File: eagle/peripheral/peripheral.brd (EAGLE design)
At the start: 160 x 100 mm, 0 parts

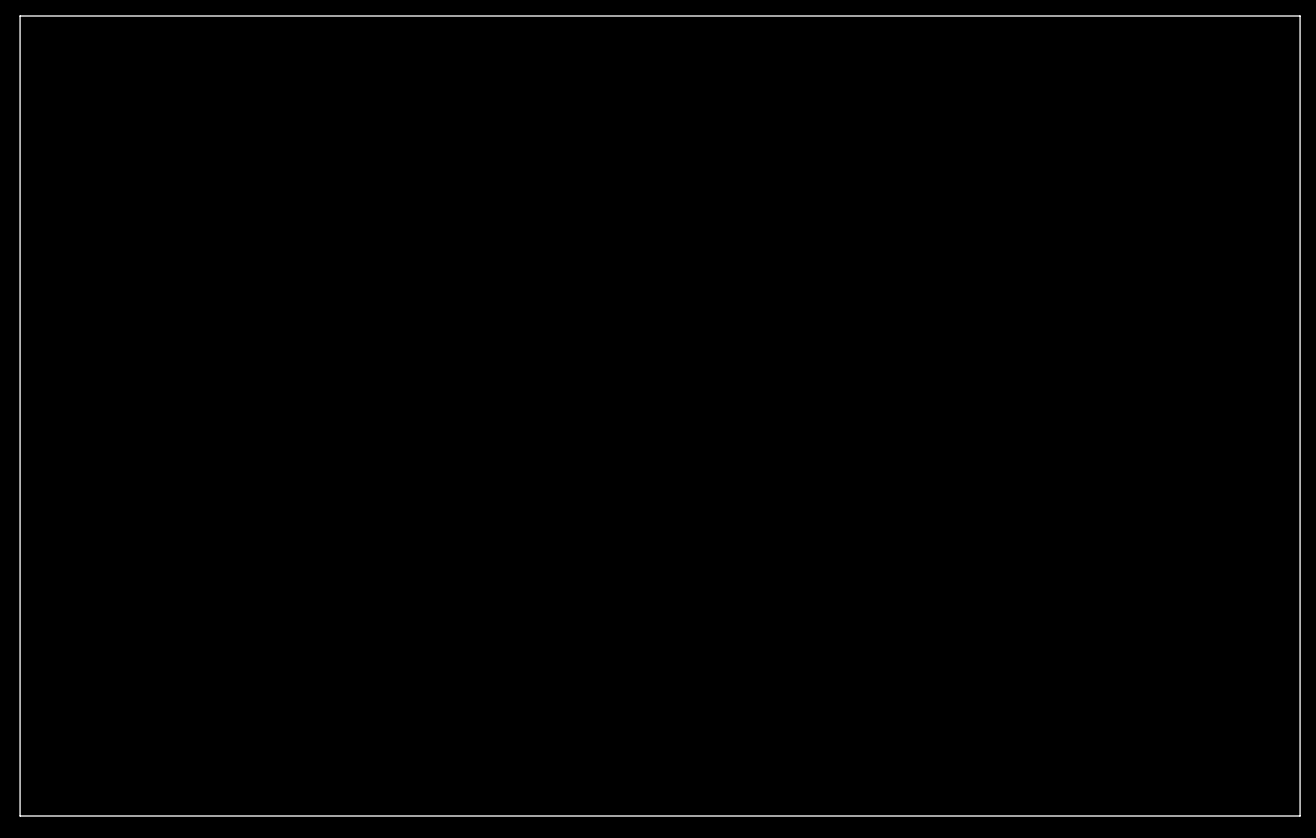
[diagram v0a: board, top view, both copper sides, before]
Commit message: Completed peripheral design layout.
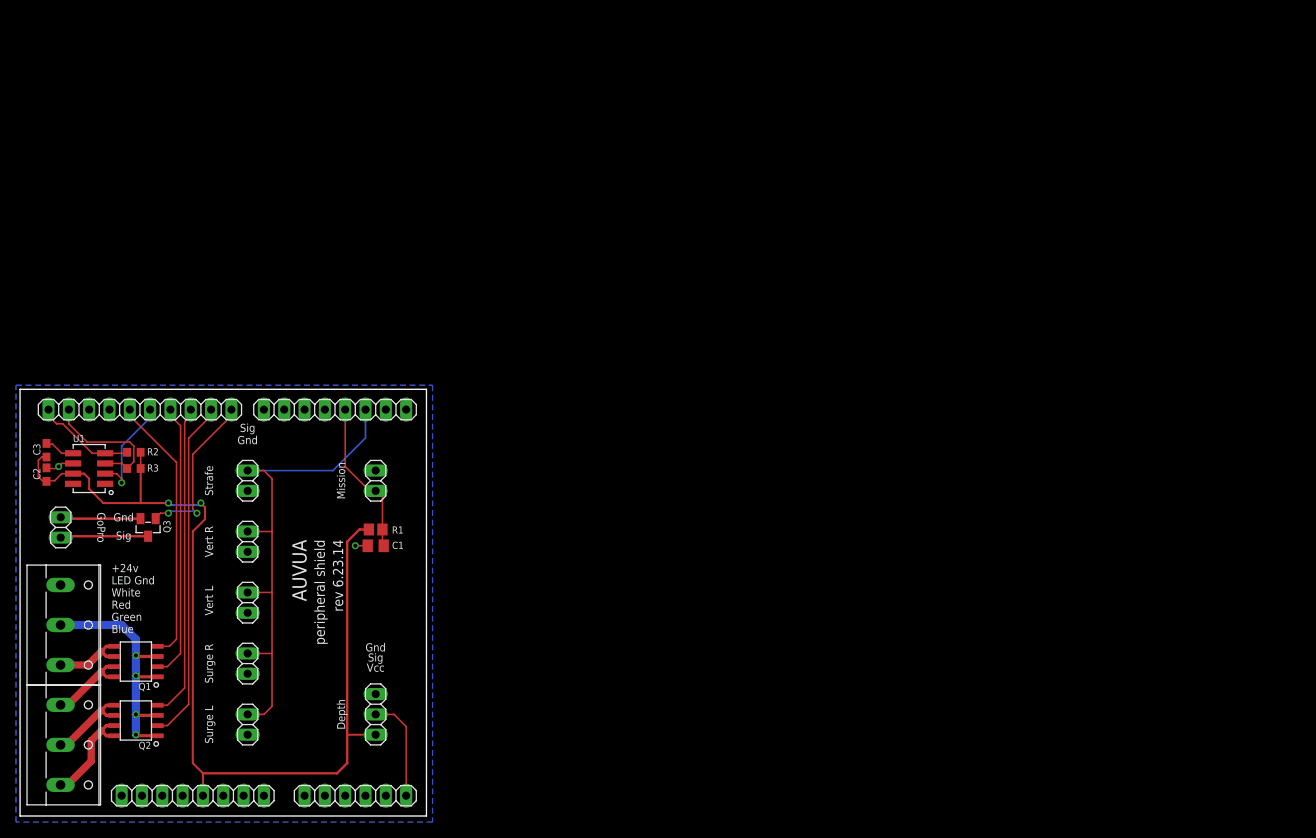
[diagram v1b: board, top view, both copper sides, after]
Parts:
- added C1: 10u, resistor:C0805K
- added C2: 220n, resistor:C0603
- added C3: 100n, resistor:C0603
- added JP1: (no value), pinhead:1X10
- added JP10, JP11, JP5, JP6, JP7, JP8, JP9: (no value), pinhead:1X02
- added JP12: (no value), pinhead:1X03
- added JP2, JP3: (no value), pinhead:1X08
- added JP4: (no value), pinhead:1X06
- added Q1, Q2: DMN4031SSD, peripheral:SO-8
- added Q3: BSS123, peripheral:SOT-23
- added R1: 100k, resistor:R0805
- added R2, R3: 4.7k, resistor:R0603
- added U1: CHIPCAP2, peripheral:CHIPCAP2
- added X1, X2: (no value), con-wago-500:W237-103
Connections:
- new net +24V: X1.1
- new net 0/RX1: JP2.8
- new net 1/TX1: JP2.7
- new net 10: JP1.8, Q2.4
- new net 11: JP1.7, Q1.2
- new net 12: JP1.6, U1.2
- new net 13: JP1.5, Q1.4
- new net 2: JP10.1, JP2.6, JP6.1, JP7.1, JP8.1, JP9.1
- new net 3: C1.1, JP2.5, JP5.1, R1.1
- new net 3.3V: JP3.4
- new net 4: JP2.4
- new net 5: JP2.3
- new net 5V: C2.1, C3.1, JP12.1, JP3.5, R1.2, R2.2, R3.2, U1.7
- new net 6: JP2.2
- new net 7: JP2.1
- new net 8: JP1.10, Q3.1
- new net 9: JP1.9, Q2.2
- new net A0: JP4.1
- new net A1: JP4.2
- new net A2: JP4.3
- new net A3: JP4.4
- new net A4: JP4.5
- new net A5: JP12.2, JP4.6
- new net AREF: JP1.3
- new net BLUE_LED: Q2.7, Q2.8, X2.3
- new net GND: C1.2, C2.2, JP1.4, JP10.2, JP11.2, JP12.3, JP3.6, JP3.7, JP5.2, JP6.2, JP7.2, JP8.2, JP9.2, Q3.3, U1.6
- new net GREEN_LED: Q2.5, Q2.6, X2.2
- new net IOREF: JP3.2
- new net N$2: JP11.1, Q3.2
- new net N$3: C3.2, U1.5
- new net N$6: Q1.1, Q1.3, Q2.1, Q2.3, X1.2
- new net RED_LED: Q1.7, Q1.8, X2.1
- new net RESET: JP3.3
- new net SCL: JP1.1, R2.1, U1.4
- new net SDA: JP1.2, R3.1, U1.3
- new net VIN: JP3.8
- new net WHITE_LED: Q1.5, Q1.6, X1.3
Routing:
- net 5V: track 0.00 -> 124.1 mm, vias 0 -> 2
- net 2: track 0.00 -> 64.5 mm
- net 9: track 0.00 -> 43.0 mm
- net 10: track 0.00 -> 39.4 mm
- net 11: track 0.00 -> 34.6 mm
- net 13: track 0.00 -> 33.9 mm
- net N$6: track 0.00 -> 33.1 mm, vias 0 -> 4
- net 8: track 0.00 -> 20.8 mm, vias 0 -> 2
- net 3: track 0.00 -> 19.8 mm
- net SDA: track 0.00 -> 17.2 mm
- net GND: track 0.00 -> 15.2 mm, vias 0 -> 2
- net 12: track 0.00 -> 13.5 mm, vias 0 -> 1
- net BLUE_LED: track 0.00 -> 13.2 mm
- net A5: track 0.00 -> 13.1 mm
- net SCL: track 0.00 -> 12.6 mm
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- added copper zone on layer 16, net GND
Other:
- board size 160 x 100 mm -> 50.8 x 53.3 mm
- board text added: "+24v"
- board text added: "AUVUA"
- board text added: "Blue"
- board text added: "Depth"
- board text added: "Gnd"
- board text added: "GoPro"
- board text added: "Green"
- board text added: "LED Gnd"
- board text added: "Mission"
- board text added: "Red"
- board text added: "Sig"
- board text added: "Strafe"
- board text added: "Surge L"
- board text added: "Surge R"
- board text added: "Vcc"
- board text added: "Vert L"
- board text added: "Vert R"
- board text added: "White"
- board text added: "peripheral shield"
- board text added: "rev 6.23.14"
